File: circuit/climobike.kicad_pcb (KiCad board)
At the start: 2 copper layers, 159 x 58 mm, 12 parts, among them IC1 ESP32-DevKitC, J1 Jack-DC, U1 DHT22, U2 Tiny_RTC_DS1307

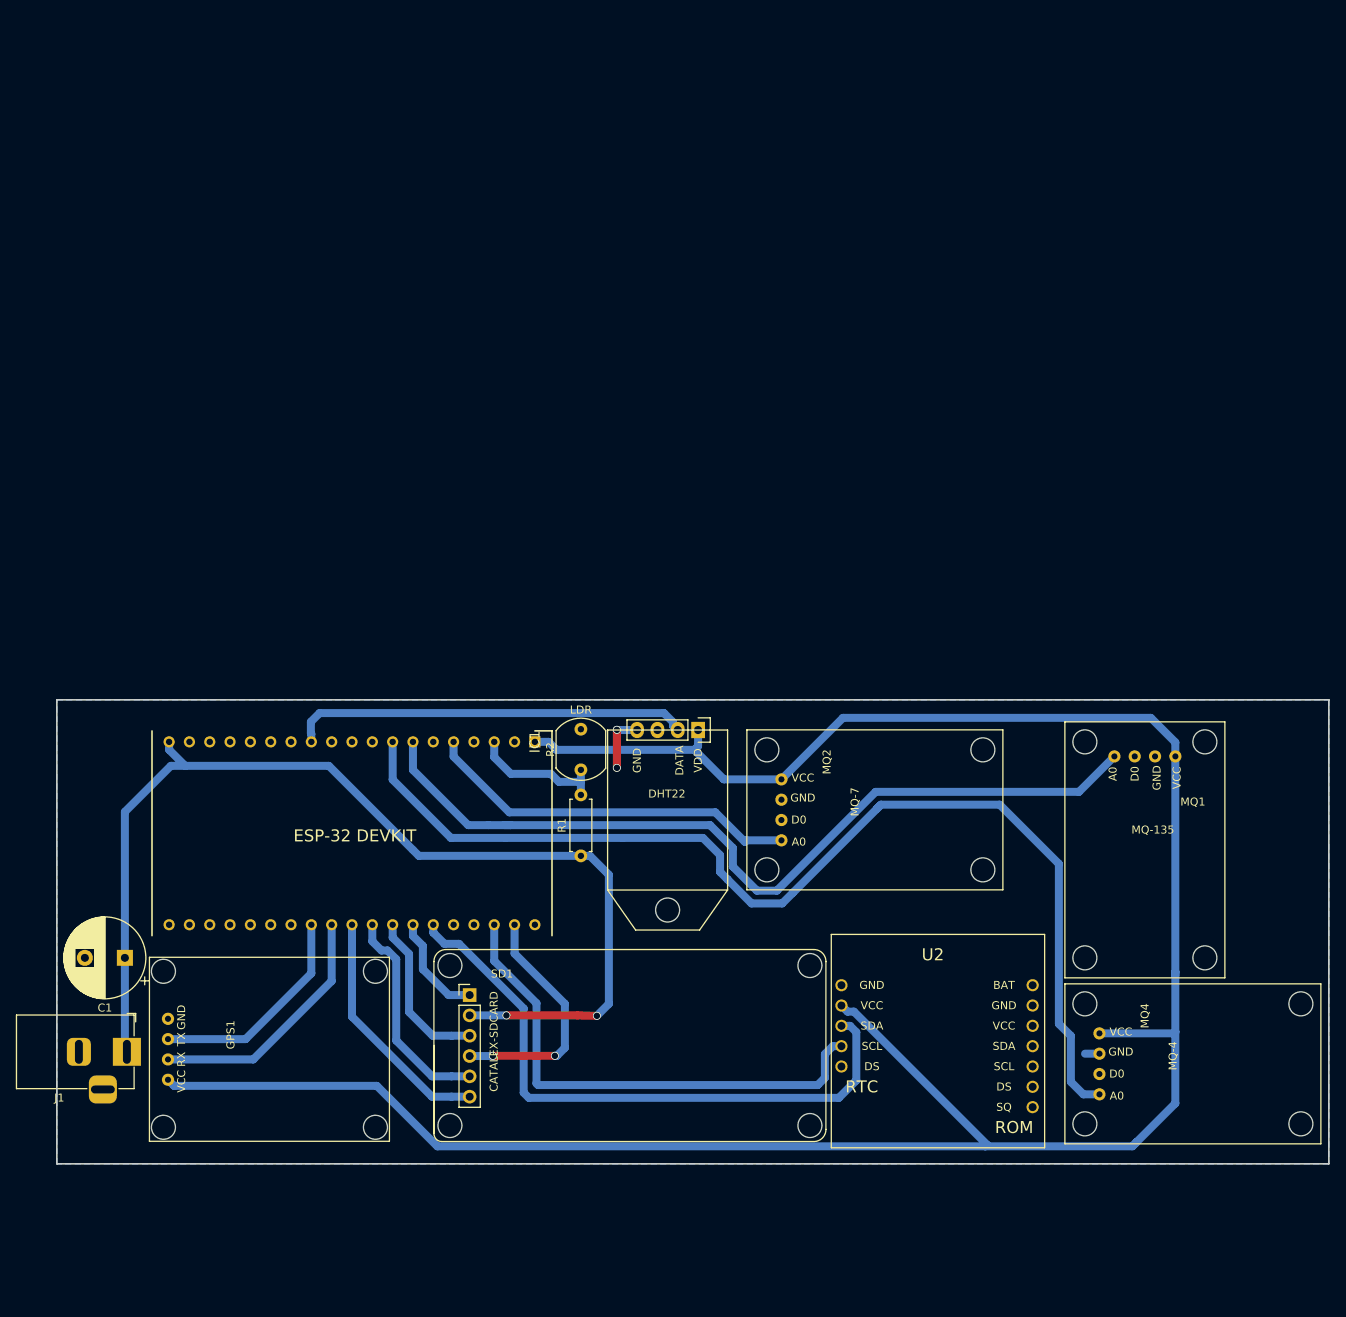
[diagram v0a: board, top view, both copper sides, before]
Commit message: ADD: Fabrication files
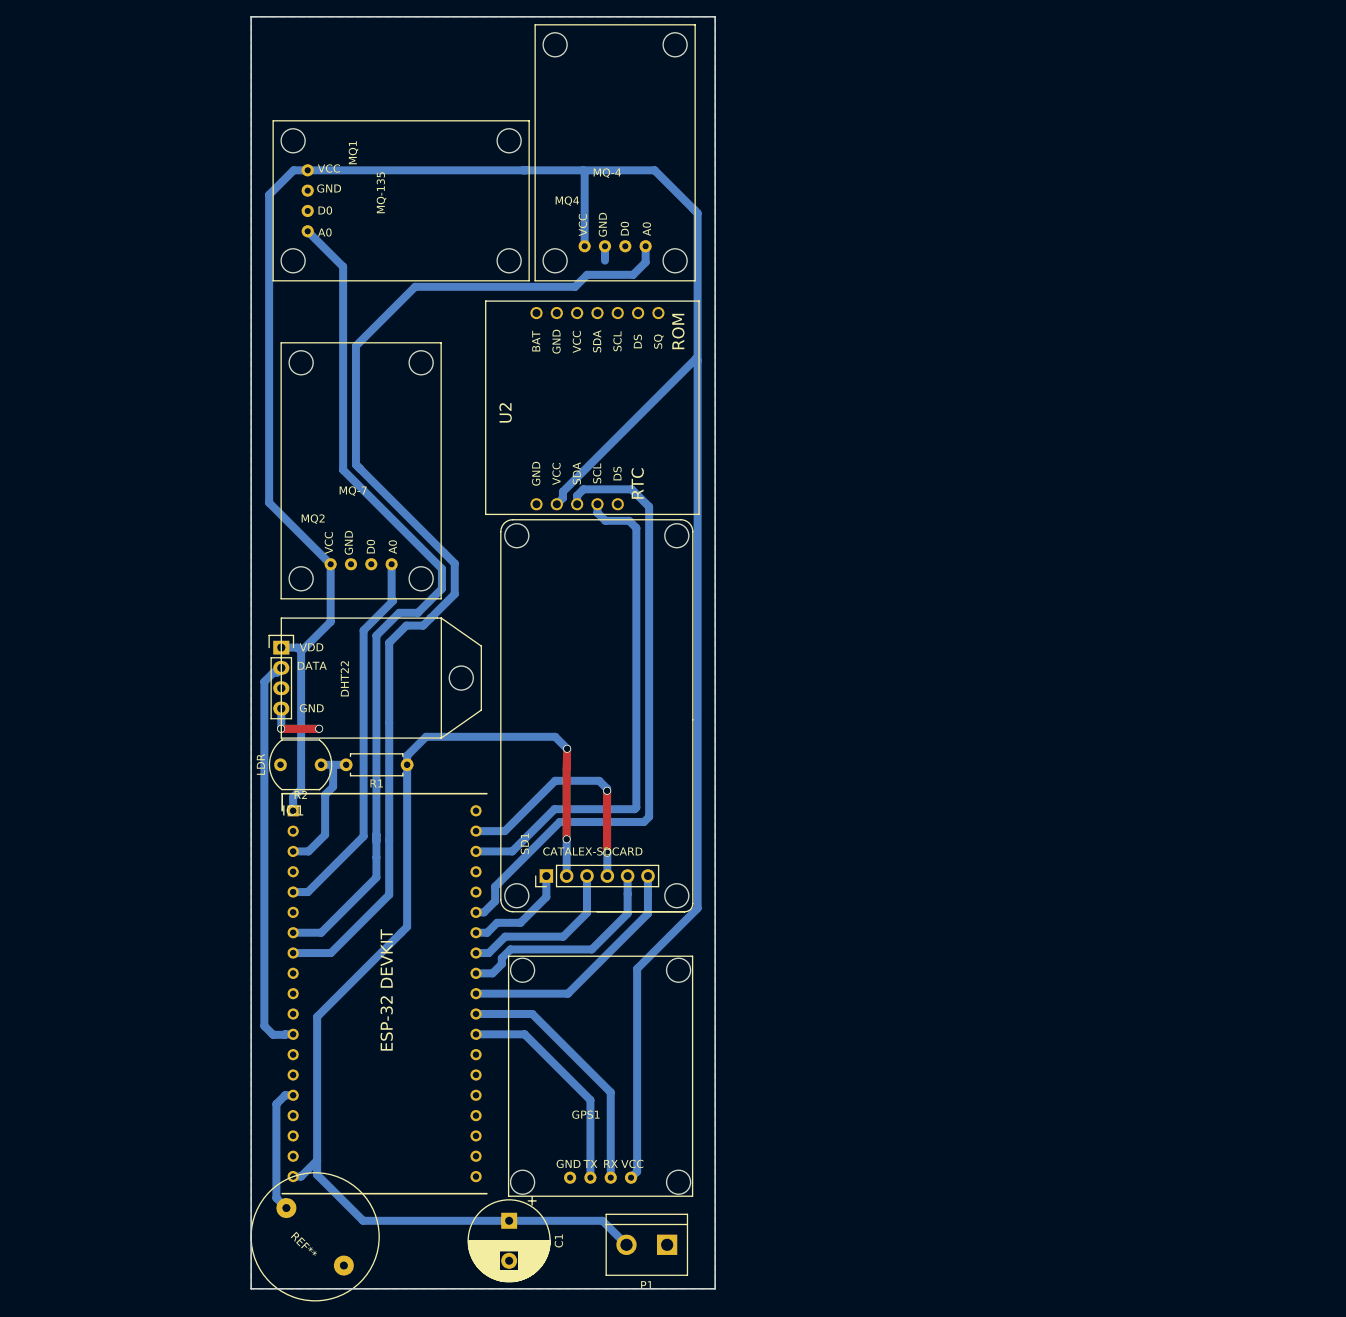
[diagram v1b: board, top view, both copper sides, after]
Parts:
- removed J1: Jack-DC, Connector_BarrelJack:BarrelJack_Horizontal
- added P1: INPUT, Connect:bornier2, F.Cu at (154.7, 160.1)
- added REF**: BUZZER, Buzzers_Beepers:BUZZER, F.Cu at (113.3, 159.1)
- moved MQ1 126.9 mm to (108.0, 29.6), turned to 270 degrees
- moved MQ4 112.9 mm to (150.8, 39.6), turned to 0 degrees
- moved U2 88.6 mm to (146.0, 56.1), turned to 270 degrees
- moved GPS1 60.6 mm to (151.0, 154.0), turned to 0 degrees
- moved C1 58.2 mm to (137.5, 157.1), turned to 270 degrees
- moved MQ2 55.0 mm to (119.0, 79.4), turned to 0 degrees
- moved U1 48.7 mm to (109.1, 89.3), turned to 270 degrees
- moved R2 32.5 mm to (114.0, 100.1), turned to 180 degrees
- moved IC1 31.4 mm to (110.5, 105.9), turned to 0 degrees
- moved SD1 26.4 mm to (148.5, 118.4), turned to 0 degrees
- moved R1 24.5 mm to (124.8, 100.1), turned to 180 degrees
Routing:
- net Net-(IC1-Pad15): track 0.00 -> 16.1 mm
- net VCC: track 136.6 -> 140.7 mm
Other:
- board size 159 x 58 mm -> 58 x 159 mm
